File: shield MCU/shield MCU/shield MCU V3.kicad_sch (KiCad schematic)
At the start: 16 parts, among them J1 IR_sensor, J2 IR_sensor, J3 IR_sensor, J4 IR_sensor, J5 IR_sensor, J6 BATT, SW1 Pwr_Sw, U1 pwr_mgr_1, U3 gy50, U4 NUCLEO144-F429ZI

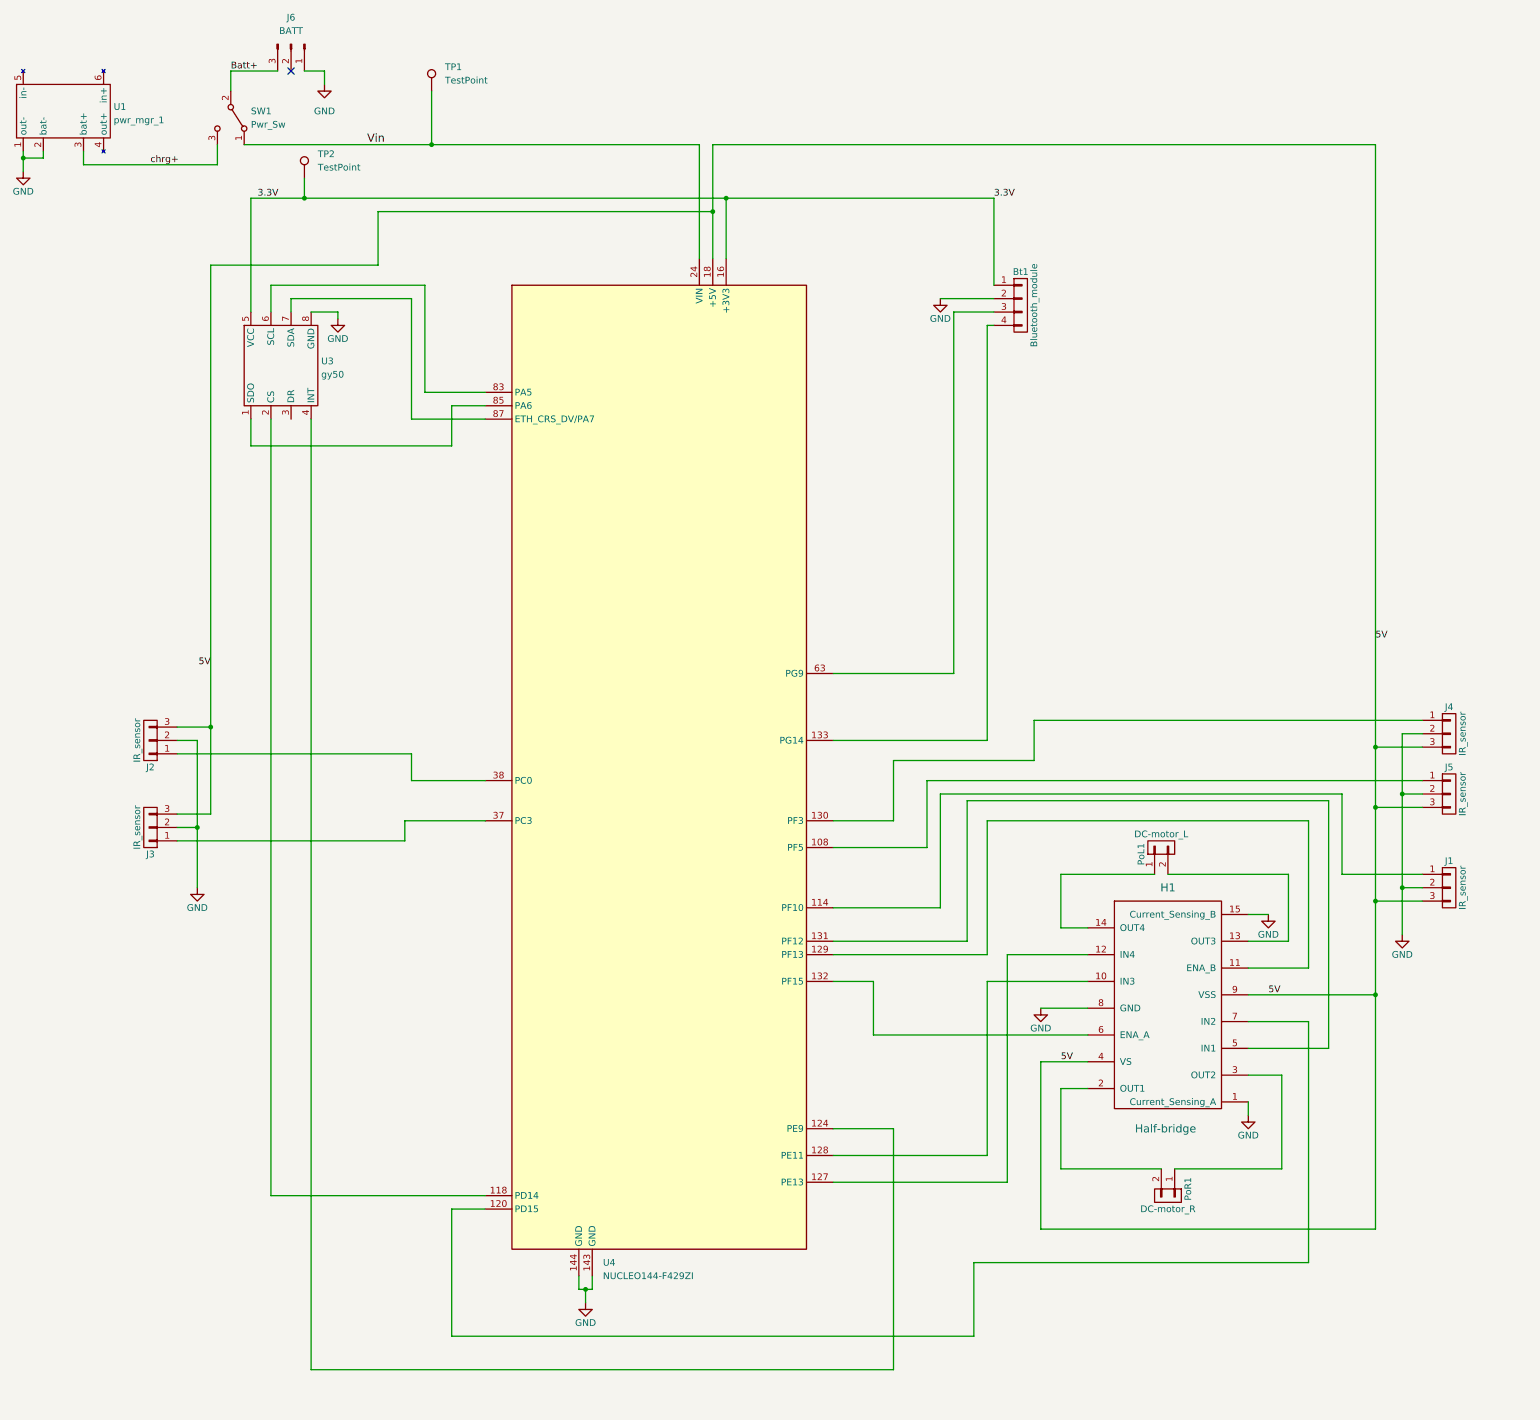
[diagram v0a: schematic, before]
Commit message: Viimeinen versio
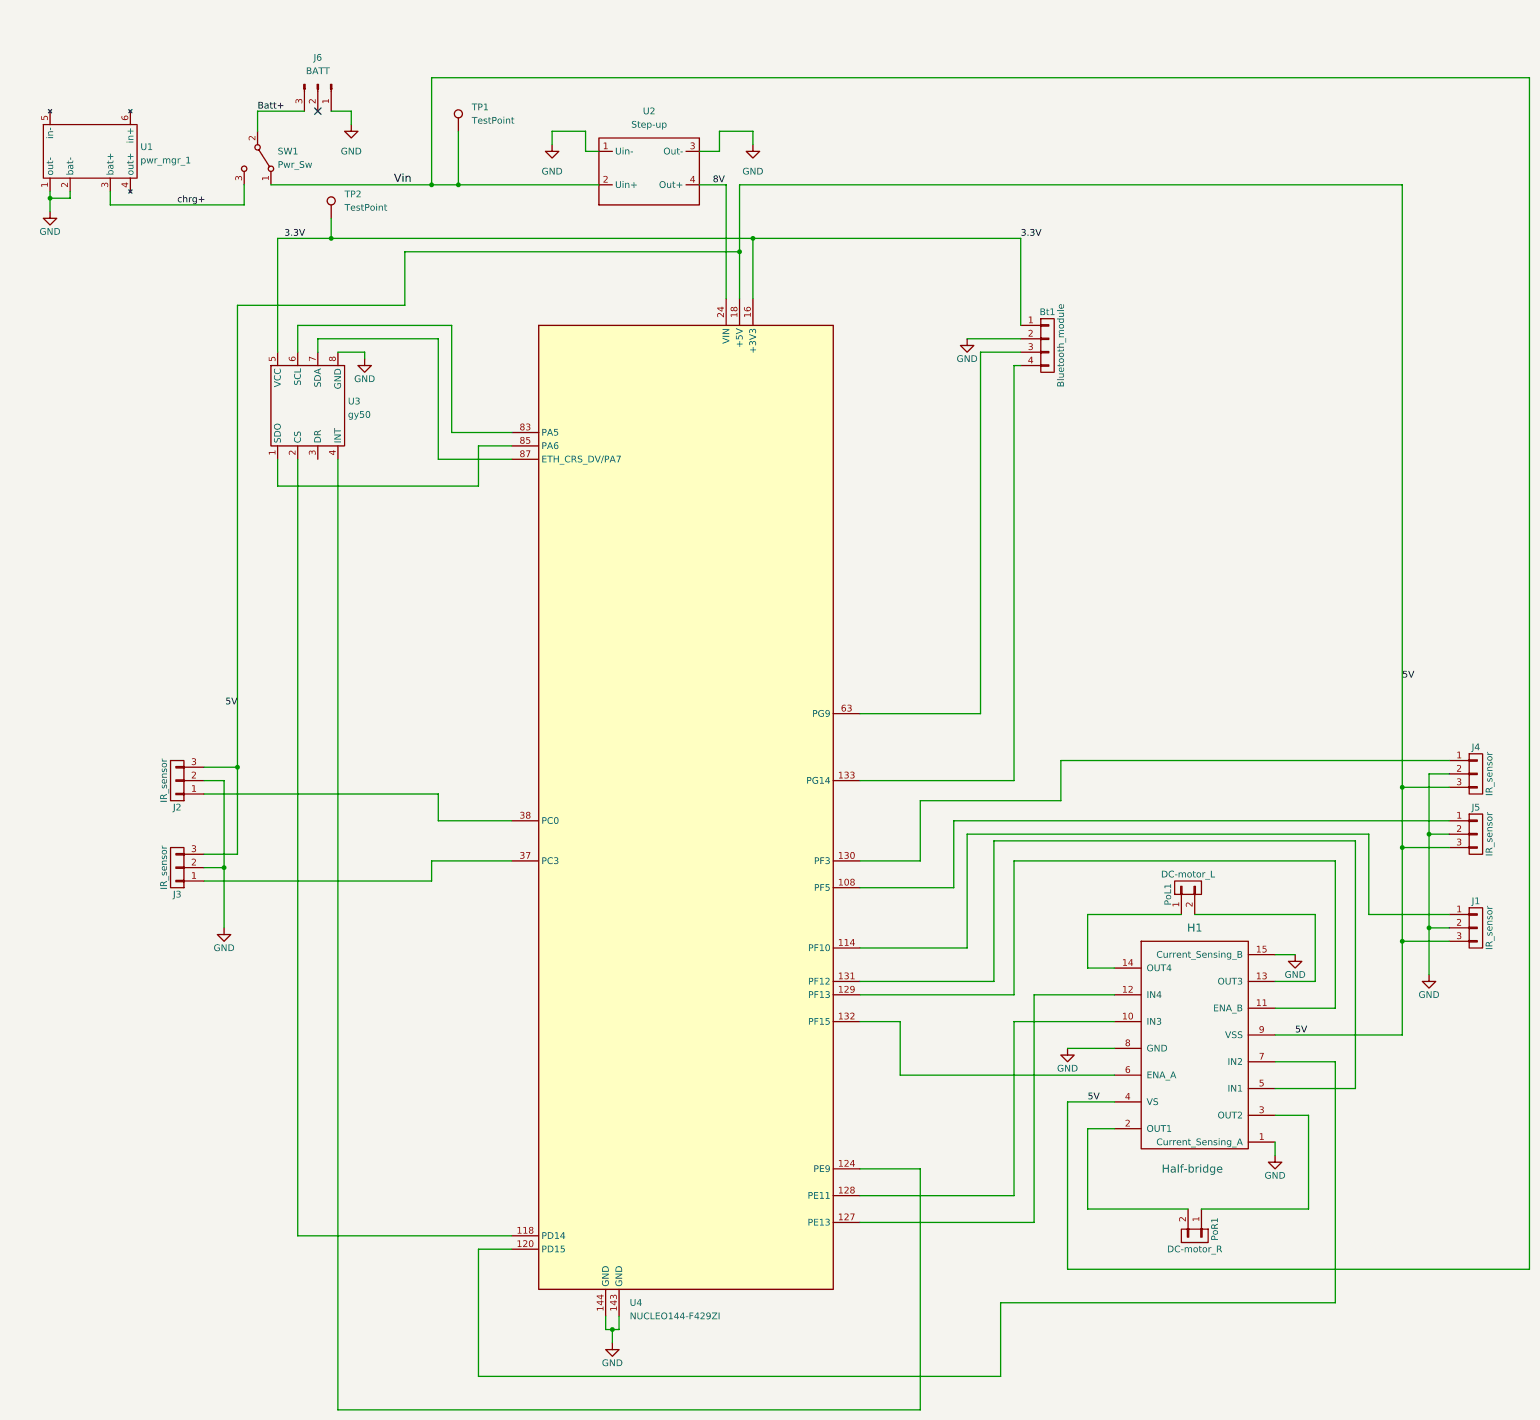
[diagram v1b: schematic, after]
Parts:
- added U2: Step-up, symbol New_Library:Step-up
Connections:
- net 5V: now also SW1.1 (A), TP1.1, U2.2 (Uin+)
- net GND: now also U2.1 (Uin-), U2.3 (Out-)
- removed net Vin: SW1.1 (A), TP1.1, U4.24 (VIN)
- new net 8V: U2.4 (Out+), U4.24 (VIN)
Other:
- moved on the sheet: Bt1, H1, J1, J2, J3, J4, J5, J6, PoL1, PoR1, SW1, TP1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
